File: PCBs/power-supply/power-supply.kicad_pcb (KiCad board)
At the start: 2 copper layers, 135 x 135 mm, 52 parts, among them J1 250V-A, J10 0V, J11 +310V-L, J12 0V, J13 +42V, J14 +42V, J15 0V, J16 0V, J17 +38V, J18 +38V, J19 0V, J2 250V-B, J20 0V, J21 -38V, J22 -38V, J3 30V-A, J4 30V-B, J5 28V-A, J6 28V-B, J7 28V-C, J8 28V-D, J9 +310V-R, U3 TL783

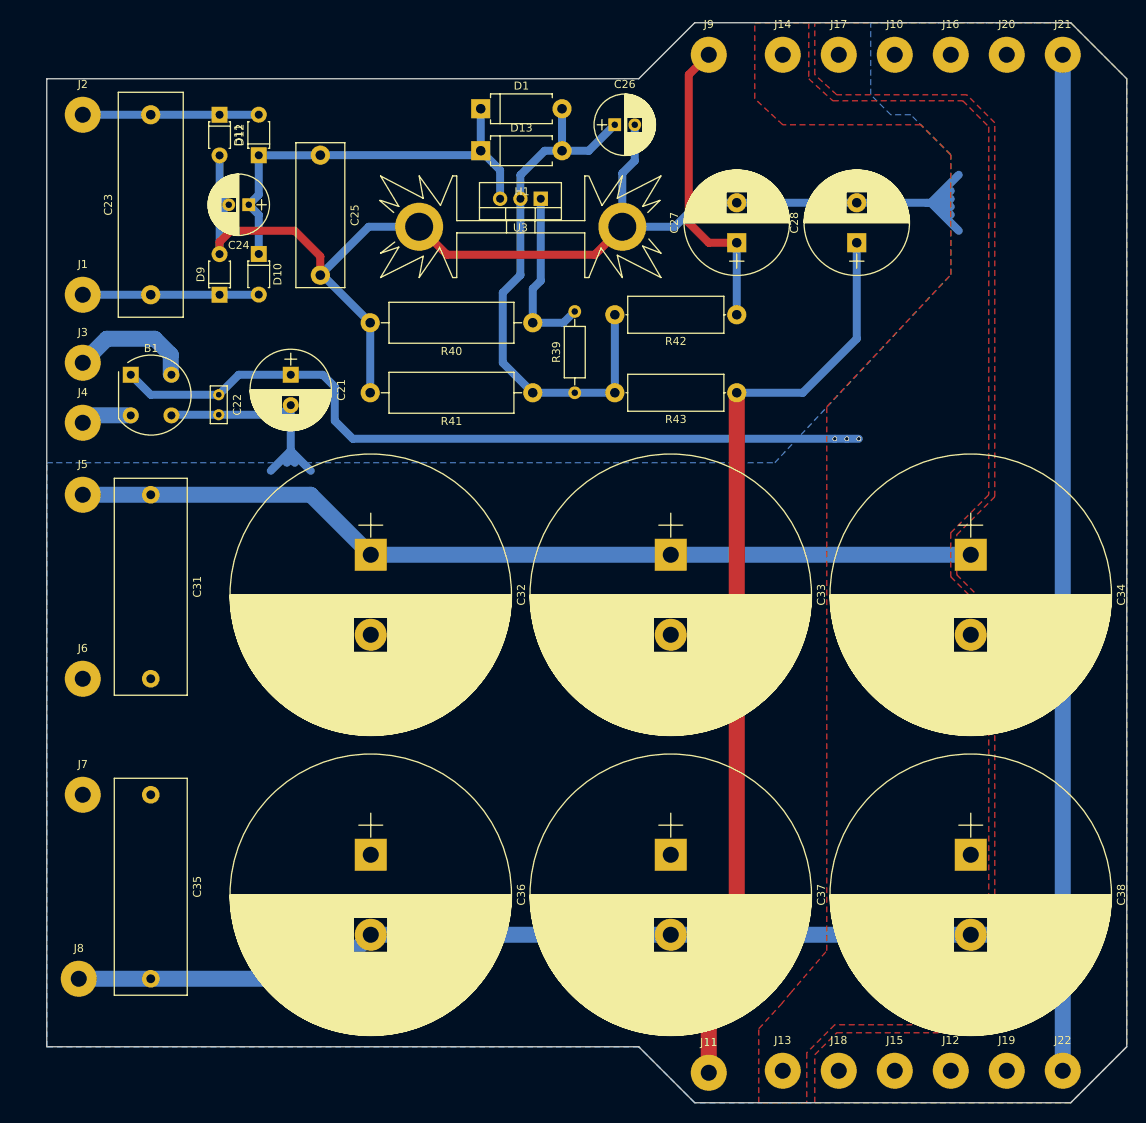
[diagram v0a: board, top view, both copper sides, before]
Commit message: Small change.
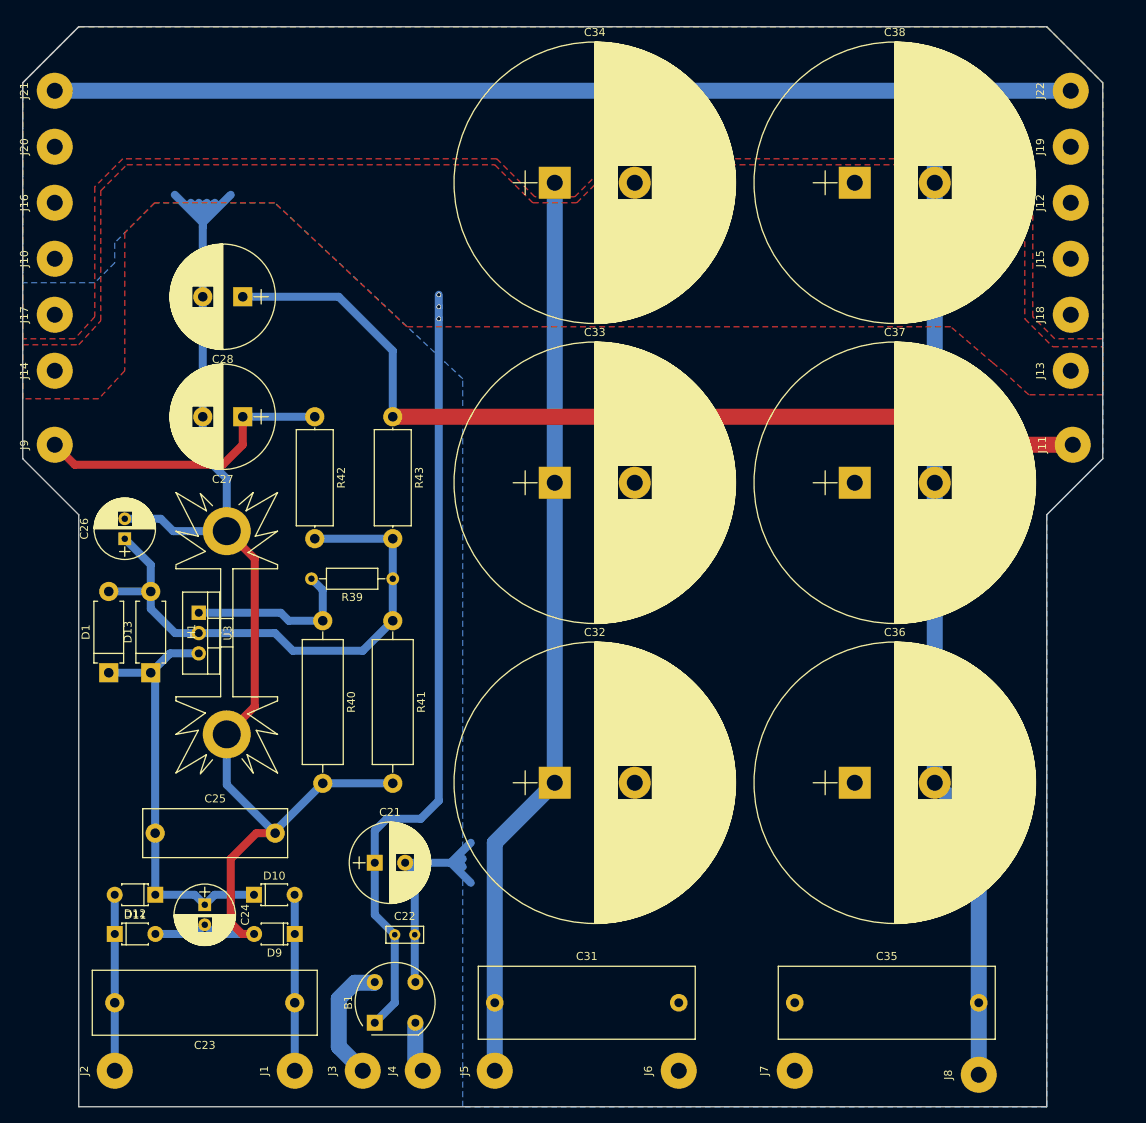
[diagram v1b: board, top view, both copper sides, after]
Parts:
- moved J21 126.1 mm to (33.0, 34.5), turned to 90 degrees
- moved J22 122.5 mm to (160.0, 34.5), turned to 90 degrees
- moved J2 119.6 mm to (40.5, 157.0), turned to 90 degrees
- moved J20 119.6 mm to (33.0, 41.5), turned to 90 degrees
- moved J19 115.8 mm to (160.0, 41.5), turned to 90 degrees
- moved J16 113.5 mm to (33.0, 48.5), turned to 90 degrees
- moved J8 113.1 mm to (148.5, 157.5), turned to 90 degrees
- moved J12 109.5 mm to (160.0, 48.5), turned to 90 degrees
- moved J10 108.1 mm to (33.0, 55.5), turned to 90 degrees
- moved J15 103.9 mm to (160.0, 55.5), turned to 90 degrees
- moved J17 103.2 mm to (33.0, 62.5), turned to 90 degrees
- moved D11 103.2 mm to (40.5, 139.9), turned to 0 degrees
- moved J1 100.6 mm to (63.0, 157.0), turned to 90 degrees
- moved J14 99.2 mm to (33.0, 69.5), turned to 90 degrees
- moved J18 98.8 mm to (160.0, 62.5), turned to 90 degrees
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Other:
- outline, holes or cut-outs redrawn
